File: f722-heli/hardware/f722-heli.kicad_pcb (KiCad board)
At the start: 6 copper layers, 41.7 x 25.4 mm, 156 parts, among them J1 USB4145-03-0170-C, J10 PORT B / JST GH, J11 PORT C / JST GH, J12 DSM / JST ZH, J2 S1 / GND-VX-S, J3 S2 / GND-VX-S, J4 S3 / GND-VX-S, J5 TAIL / GND-VX-S, J6 ESC / GND-VX-S, J7 RPM / GND-VX-S, J8 SBUS / GND-VX-S, J9 PORT A / JST GH, Q1 BSS138LT1G, Q2 BSS138LT1G, SW1 BOOT / KMT031NGJLHS, U1 STM32F722RET6, U10 TPS2553DRVR / USB input limit, U11 TPS2553DRVR / DSM output limit, U12 USBLC6-4SC6 / header clamp, U13 USBLC6-4SC6 / header clamp, U14 TPD4E05U06DQAR / UART ESD, U15 TPD4E05U06DQAR / UART ESD, U16 PESD15VS2UT,215 / 15V ESD, U2 ICM-42688-P, U3 W25N01GVZEIG / 128MiB, U4 DPS368XTSA1 / 0x76, U5 TPS259472ARPWR, U6 TPS63070RNMR / nominal 5.088V, U7 TPS2117DRLR / ABC priority mux, U8 TPS2121RUXR / BEC-priority co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, U9 TPS62162DSGR / 3.3V 1A, Y1 8MHz / CL10pF / TAXM8M4RDBCCT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

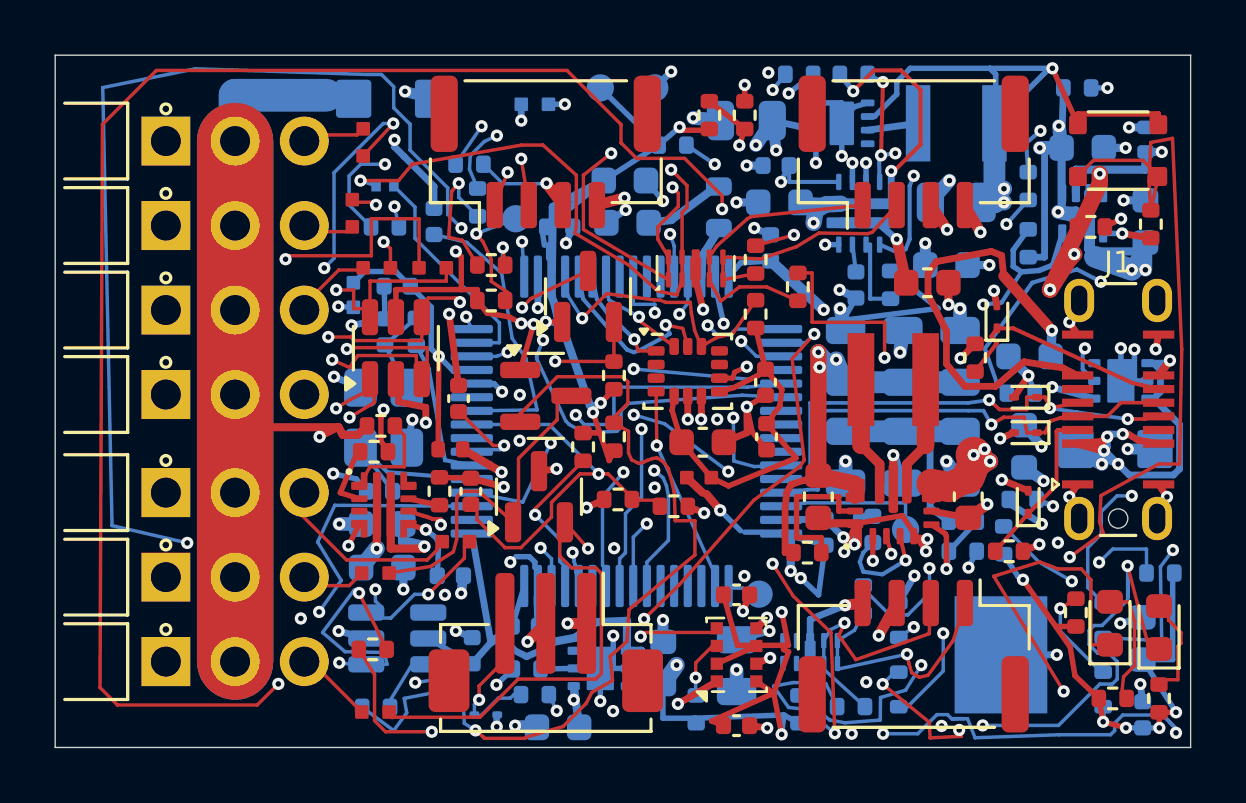
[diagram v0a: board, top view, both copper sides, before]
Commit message: cleaned up the nets
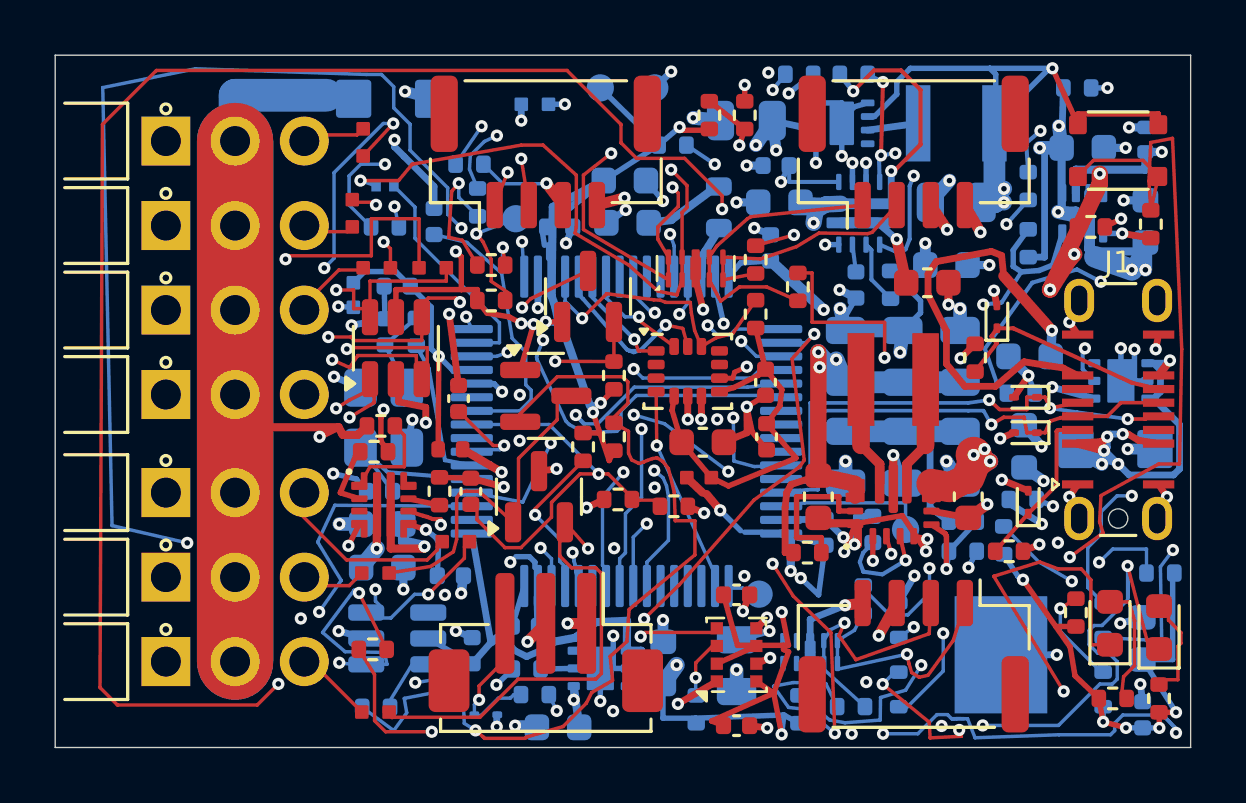
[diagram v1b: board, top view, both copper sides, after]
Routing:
- net IMU_MISO: track 3.96 -> 4.70 mm
- net GND: track 133.7 -> 133.0 mm
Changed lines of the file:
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@@
 	)
 	(segment
+		(start 31.75 9.015)
+		(end 31.75 9.45)
+		(width 0.2)
+		(layer "B.Cu")
+		(net "GND")
+	)
+	(segment
+		(start 29 10.1)
+		(end 31.1 10.1)
+		(width 0.5)
+		(layer "B.Cu")
+		(net "GND")
+	)
+	(segment
 		(start 30.95 20.095)
 		(end 31.525 19.0991)
@@
 	)
 	(segment
-		(start 32.396952 9.29107)
-		(end 28.906761 9.72849)
-		(width 0.2)
-		(layer "B.Cu")
-		(net "GND")
-	)
-	(segment
 		(start 34.975 11.05)
 		(end 35.7078 11.7601)
@@
 	)
 	(segment
+		(start 31.75 9.45)
+		(end 31.1 10.1)
+		(width 0.2)
+		(layer "B.Cu")
+		(net "GND")
+	)
+	(segment
 		(start 15.2 4.186072)
 		(end 15.230688 3.682091)
@@
 	)
 	(segment
-		(start 30.65 7.915)
-		(end 32.396952 9.29107)
-		(width 0.2)
-		(layer "B.Cu")
-		(net "GND")
-	)
-	(segment
 		(start 14.98 19.1)
 		(end 14.8952 19.7444)
@@
 	)
 	(segment
+		(start 30.65 7.915)
+		(end 31.75 9.015)
+		(width 0.2)
+		(layer "B.Cu")
+		(net "GND")
+	)
+	(segment
 		(start 29 15.7)
 		(end 29 14.9)
@@
 	)
 	(segment
-		(start 25.209999 12.475)
-		(end 21.034999 12.775)
+		(start 21.034999 12.775)
+		(end 21.325499 12.4845)
+		(width 0.127)
+		(layer "B.Cu")
+		(net "PORT_B_TX_MCU")
+	)
+	(segment
+		(start 21.325499 12.4845)
+		(end 26.569499 12.4845)
 		(width 0.127)
 		(layer "B.Cu")
@@
 	)
 	(segment
-		(start 26.634999 12.55)
-		(end 25.209999 12.475)
+		(start 26.569499 12.4845)
+		(end 26.634999 12.55)
 		(width 0.127)
 		(layer "B.Cu")
@@
 	(segment
 		(start 25.4 12.18)
-		(end 20.5 12.18)
+		(end 21.248938 12.18)
 		(width 0.127)
 		(layer "B.Cu")
@@
 	)
 	(segment
-		(start 20.5 13.55)
-		(end 19.4 13.55)
+		(start 19.425619 13.525619)
+		(end 19.903319 13.525619)
 		(width 0.127)
 		(layer "B.Cu")
@@
 	)
 	(segment
-		(start 20.5 12.18)
-		(end 20.5 13.55)
+		(start 19.1 13.2)
+		(end 19.425619 13.525619)
 		(width 0.127)
 		(layer "B.Cu")
@@
 	)
 	(segment
+		(start 19.903319 13.525619)
+		(end 21.248938 12.18)
+		(width 0.127)
+		(layer "B.Cu")
+		(net "PORT_B_RX_MCU")
+	)
+	(segment
 		(start 21.996687 11.652784)
 		(end 24.865539 10.153233)
@@
 	)
 	(segment
-		(start 18.809999 8.825)
-		(end 18.709999 8.125)
+		(start 18.709999 8.125)
+		(end 18.709999 9.025)
 		(width 0.127)
 		(layer "B.Cu")
@@
 	)
 	(segment
-		(start 19.334999 9.65)
-		(end 18.809999 8.825)
+		(start 18.709999 9.025)
+		(end 19.334999 9.65)
 		(width 0.127)
 		(layer "B.Cu")
@@
 	)
 	(segment
-		(start 17.681092 13.013085)
-		(end 15.284999 13.05)
+		(start 13.9 6.58)
+		(end 15.104765 6.868228)
 		(width 0.127)
 		(layer "B.Cu")
@@
 	)
 	(segment
-		(start 13.9 6.58)
-		(end 15.104765 6.868228)
+		(start 17.265248 10.888842)
+		(end 16.768394 10.391988)
+		(width 0.127)
+		(layer "B.Cu")
+		(net "ADC_BUS")
+	)
+	(segment
+		(start 17.265248 12.09352)
+		(end 17.462884 12.291156)
+		(width 0.127)
+		(layer "B.Cu")
+		(net "ADC_BUS")
+	)
+	(segment
+		(start 17.265248 12.09352)
+		(end 17.265248 10.888842)
 		(width 0.127)
 		(layer "B.Cu")
@@
 	)
 	(segment
-		(start 17.265248 11.117147)
-		(end 17.681092 13.013085)
+		(start 17.462884 12.291156)
+		(end 17.462884 12.635368)
 		(width 0.127)
 		(layer "B.Cu")
@@
 	)
 	(segment
-		(start 16.768394 10.391988)
-		(end 17.265248 11.117147)
+		(start 16.4252 7.0556)
+		(end 16.554 7.1844)
+		(width 0.127)
+		(layer "B.Cu")
+		(net "ADC_BUS")
+	)
+	(segment
+		(start 17.048252 13.05)
+		(end 15.284999 13.05)
+		(width 0.127)
+		(layer "B.Cu")
+		(net "ADC_BUS")
+	)
+	(segment
+		(start 17.462884 12.635368)
+		(end 17.048252 13.05)
 		(width 0.127)
 		(layer "B.Cu")
@@
 	)
 	(segment
-		(start 21.209999 9.14)
-		(end 21.209999 8.125)
+		(start 21.209999 8.777552)
+		(end 21.882447 9.45)
 		(width 0.127)
 		(layer "B.Cu")
@@
 	)
 	(segment
-		(start 22 9.45)
-		(end 22 9.14)
+		(start 21.209999 8.125)
+		(end 21.209999 8.777552)
 		(width 0.127)
 		(layer "B.Cu")
@@
 	)
 	(segment
-		(start 22 9.14)
-		(end 21.209999 9.14)
+		(start 21.882447 9.45)
+		(end 22 9.45)
 		(width 0.127)
 		(layer "B.Cu")
@@
 	(segment
 		(start 19.709999 8.125)
-		(end 19.875 8.95)
+		(end 19.709999 8.884999)
 		(width 0.15)
 		(layer "B.Cu")
@@
 	)
 	(segment
-		(start 20.25 9.45)
+		(start 19.709999 8.884999)
 		(end 21.25 10.425)
 		(width 0.15)
@@
 	)
 	(segment
-		(start 19.875 8.95)
-		(end 20.25 9.45)
+		(start 19.709999 8.125)
+		(end 19.709999 8.784999)
 		(width 0.15)
 		(layer "B.Cu")
@@
 	)
 	(segment
-		(start 22.55 10.225)
+		(start 21.448 10.852)
 		(end 22.4 9.9)
 		(width 0.15)
@@
 	)
 	(segment
-		(start 19.209999 8.125)
-		(end 19.375 8.95)
+		(start 21.07313 10.852)
+		(end 21.448 10.852)
 		(width 0.15)
 		(layer "B.Cu")
@@
 	)
 	(segment
-		(start 21.45 10.825)
-		(end 22.55 10.225)
+		(start 19.209999 8.125)
+		(end 19.209999 8.784999)
 		(width 0.15)
 		(layer "B.Cu")
@@
 	)
 	(segment
+		(start 19.209999 8.784999)
+		(end 19.375 8.95)
+		(width 0.15)
+		(layer "B.Cu")
+		(net "IMU_SCK")
+	)
+	(segment
 		(start 21.509999 9.8)
 		(end 21.42 9.6)
@@
 	)
 	(segment
-		(start 20.309999 8.975)
-		(end 21.42 9.6)
+		(start 20.209999 8.899999)
+		(end 20.91 9.6)
+		(width 0.127)
+		(layer "B.Cu")
+		(net "IMU_MOSI")
+	)
+	(segment
+		(start 20.209999 8.125)
+		(end 20.209999 8.899999)
 		(width 0.127)
 		(layer "B.Cu")
@@
 	)
 	(segment
-		(start 20.309999 8.975)
-		(end 20.209999 8.125)
+		(start 20.91 9.6)
+		(end 21.42 9.6)
 		(width 0.127)
 		(layer "B.Cu")
@@
 	)
 	(segment
-		(start 26.634999 11.55)
-		(end 25.712467 11.751146)
+		(start 25.547106 11.8455)
+		(end 25.842606 11.55)
 		(width 0.127)
 		(layer "B.Cu")
@@
 	)
 	(segment
-		(start 25.45 11.89)
-		(end 21.222599 11.513264)
+		(start 38.45 20.095)
+		(end 37.885022 19.530022)
 		(width 0.127)
 		(layer "B.Cu")
@@
 	)
 	(segment
-		(start 38.45 20.095)
-		(end 37.885022 19.530022)
+		(start 21.222599 11.513264)
+		(end 21.554835 11.8455)
 		(width 0.127)
 		(layer "B.Cu")
@@
 	)
 	(segment
+		(start 21.554835 11.8455)
+		(end 25.547106 11.8455)
+		(width 0.127)
+		(layer "B.Cu")
+		(net "FLASH_MOSI")
+	)
+	(segment
 		(start 37.885022 19.530022)
 		(end 37.885022 18.064978)
@@
 	)
 	(segment
-		(start 25.712467 11.751146)
-		(end 25.45 11.89)
+		(start 25.842606 11.55)
+		(end 26.634999 11.55)
 		(width 0.127)
 		(layer "B.Cu")
@@
 	)
 	(segment
-		(start 29.9 6.95)
-		(end 29.9 8.935)
+		(start 29.75 6.95)
+		(end 29.948 7.148)
+		(width 0.15)
+		(layer "B.Cu")
+		(net "CORE_ILIM")
+	)
+	(segment
+		(start 29.948 7.148)
+		(end 29.948 8.233)
 		(width 0.15)
 		(layer "B.Cu")
@@
 	)
 	(segment
-		(start 29.9 8.935)
+		(start 29.948 8.233)
 		(end 30.65 8.935)
 		(width 0.15)
@@
 	(segment
 		(start 29.75 6.95)
-		(end 29.9 6.95)
+		(end 29.892 7.092)
 		(width 0.15)
 		(layer "B.Cu")

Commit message: tidied up the nets
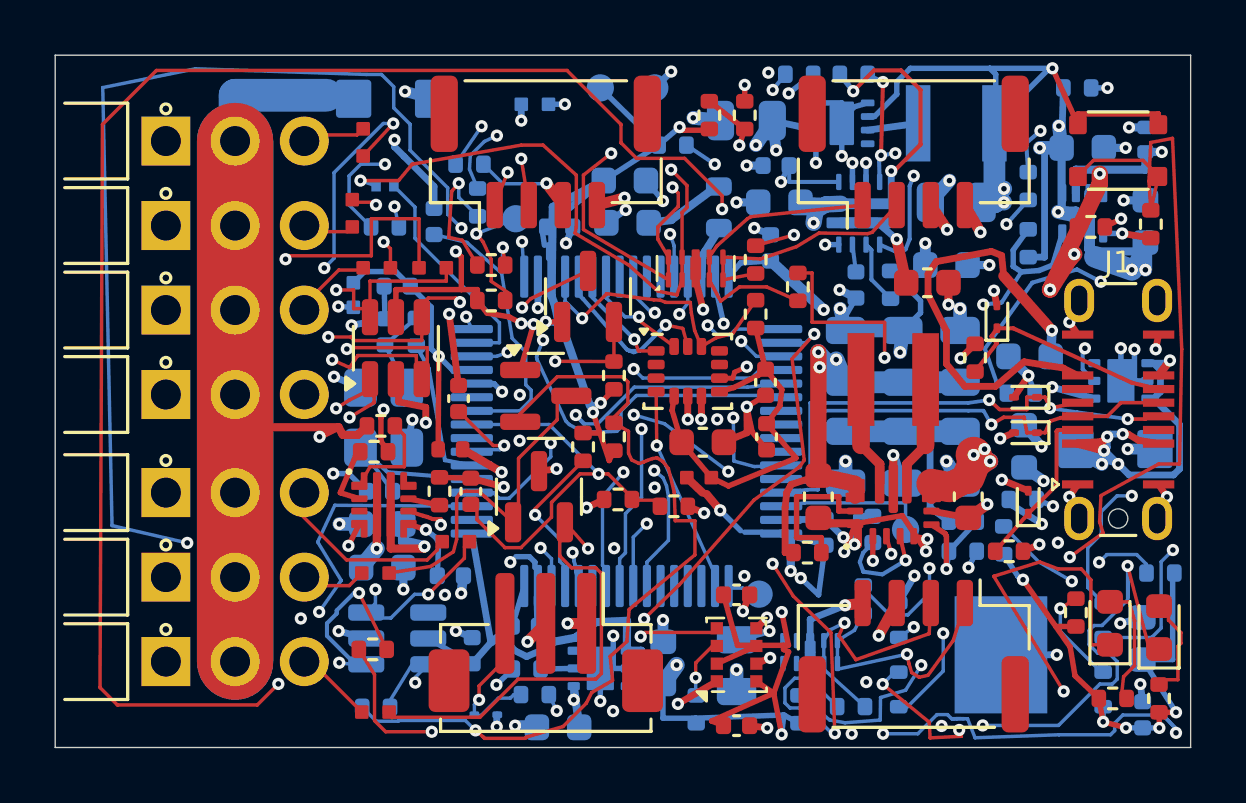
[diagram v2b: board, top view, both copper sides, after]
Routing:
- net RPM_LV: track 32.3 -> 30.1 mm
- net RPM_MCU: track 59.0 -> 57.3 mm
- net SBUS_MCU: track 51.0 -> 49.7 mm
- net PORT_C_TX_MCU: track 34.4 -> 33.9 mm
